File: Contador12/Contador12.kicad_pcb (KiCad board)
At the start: 2 copper layers, 43.2 x 38.8 mm, 17 parts, among them J1 Conector_ESP

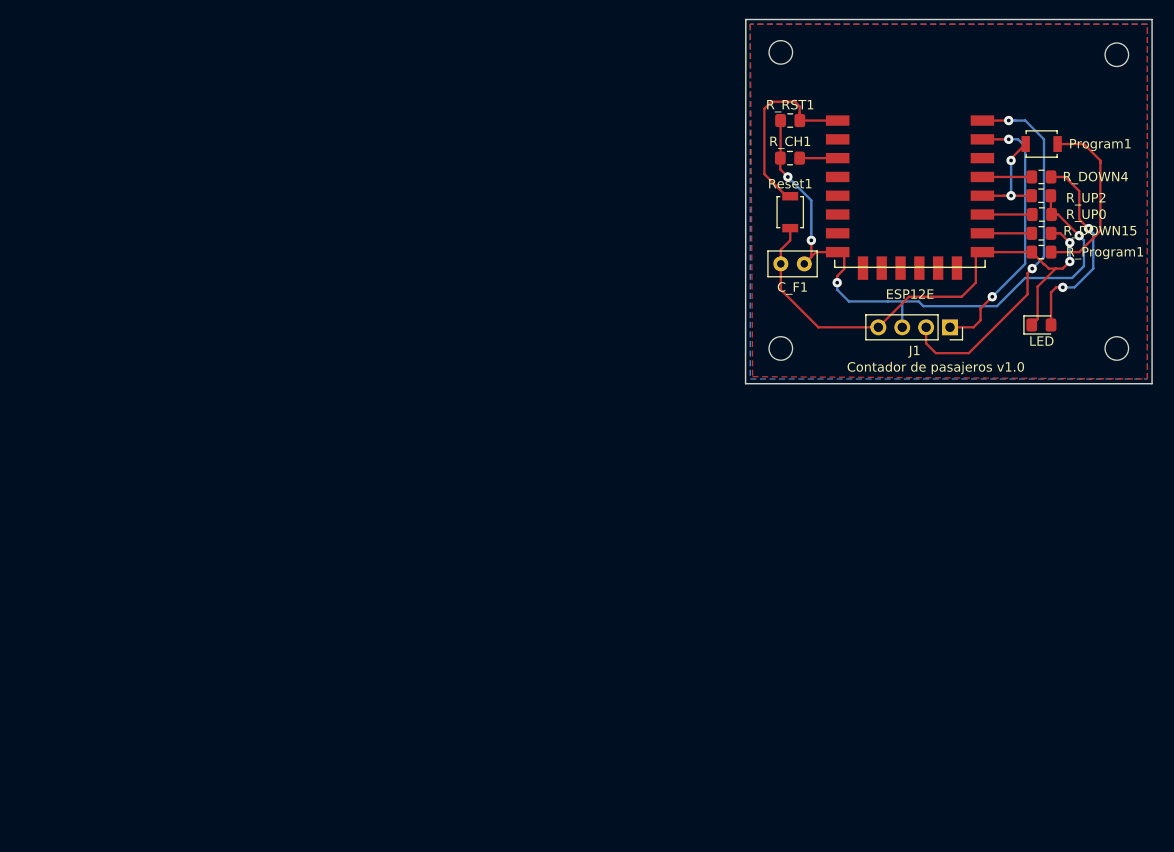
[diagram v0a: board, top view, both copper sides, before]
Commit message: Correcciones Adrian
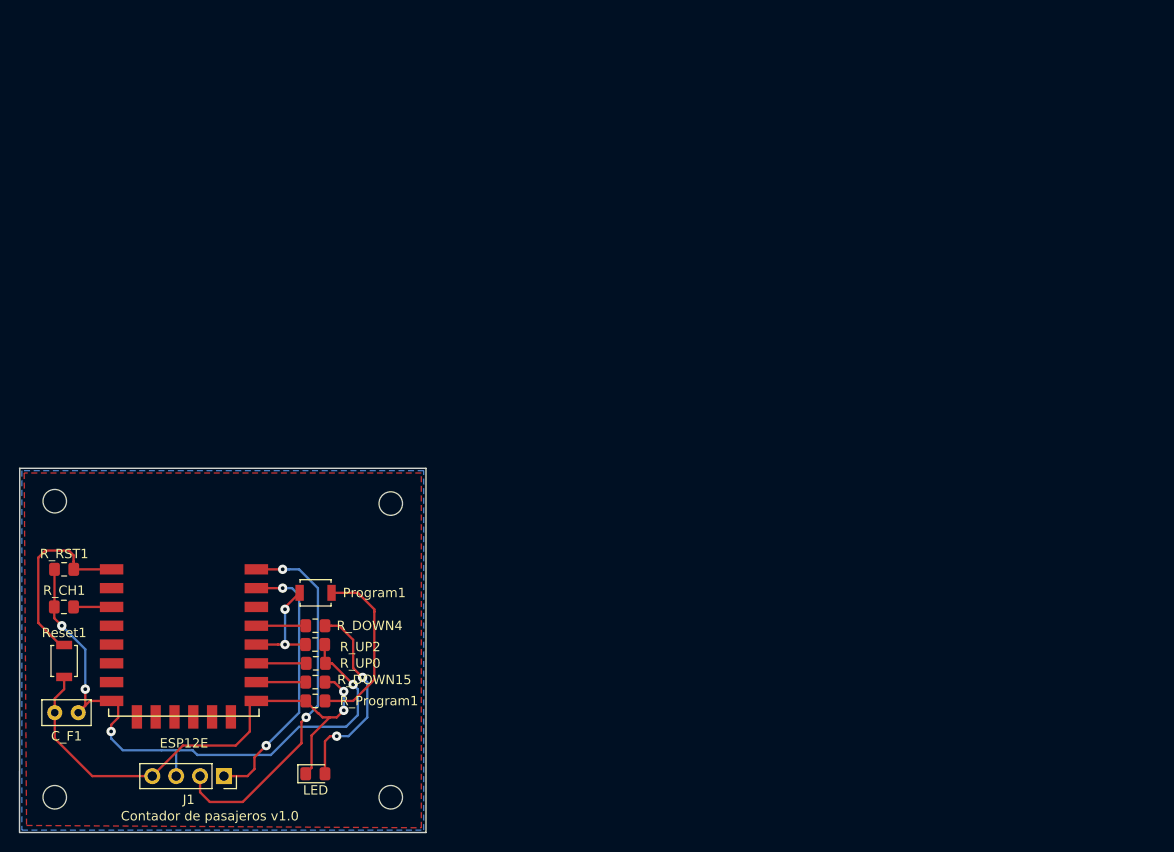
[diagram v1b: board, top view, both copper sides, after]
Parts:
- moved C_F1 90.8 mm to (105.5, 98.0)
- moved ESP12E 90.8 mm to (109.8, 82.8)
- moved J1 90.8 mm to (121.0, 104.8)
- moved LED 90.8 mm to (130.7, 104.5)
- moved MH1 90.8 mm to (103.0, 75.5)
- moved MH2 90.8 mm to (138.8, 75.8)
- moved MH3 90.8 mm to (103.0, 107.0)
- moved MH4 90.8 mm to (138.8, 107.0)
- moved Program1 90.8 mm to (130.8, 85.2)
- moved R_CH1 90.8 mm to (104.0, 86.8)
- moved R_DOWN15 90.8 mm to (130.7, 94.8)
- moved R_DOWN4 90.8 mm to (130.7, 88.8)
- moved R_Program1 90.8 mm to (130.7, 96.8)
- moved R_RST1 90.8 mm to (104.0, 82.8)
- moved R_UP0 90.8 mm to (130.7, 90.8)
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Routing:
- added copper zone on B.Cu, net +3V3
- removed copper zone on B.Cu, net GND
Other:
- board text added: "Margen: 0.25 mm Ancho pista: 0.25 mm Diametro Via: 1 mm Taladro via: 0.4 mm Cuadricula: 0.25 mm Fabricante: https://www.pcbcart.com/pcb-fab/hdi-pcb.html"
